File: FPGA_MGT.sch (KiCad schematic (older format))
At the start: 5 parts, among them U1 XC7K160T-FFG676

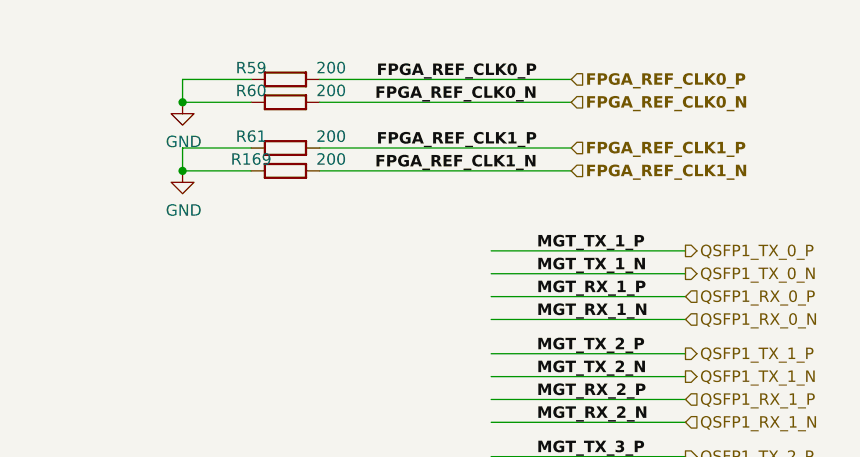
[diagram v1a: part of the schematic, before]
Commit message: REF CLK for MIG
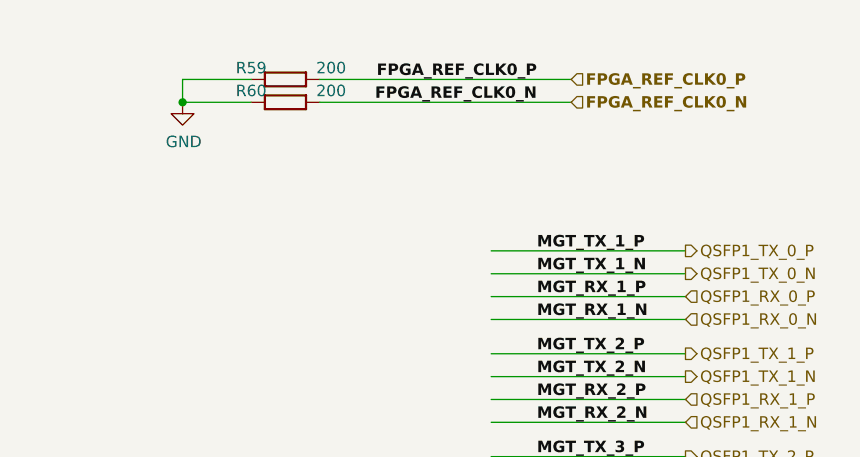
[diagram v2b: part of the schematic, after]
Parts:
- removed R169, R61: R0201_100R_1%_0.05W_200PPM, RESC0603X28N, symbol Resistors_SMD:R0201_100R_1%_0.05W_200PPM
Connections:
- net labels removed: FPGA_REF_CLK1_N, FPGA_REF_CLK1_P
- wire segments 148 -> 143
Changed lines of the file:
@@
 Comment4 ""
 $EndDescr
-Text HLabel 9700 1200 2    50   Input ~ 10
-FPGA_REF_CLK1_N
-Text HLabel 9700 1100 2    50   Input ~ 10
-FPGA_REF_CLK1_P
 Text HLabel 9700 900  2    50   Input ~ 10
 FPGA_REF_CLK0_N
@@
 Text Label 9550 900  2    50   ~ 10
 FPGA_REF_CLK0_N
-Text Label 9550 1100 2    50   ~ 10
-FPGA_REF_CLK1_P
-Text Label 9550 1200 2    50   ~ 10
-FPGA_REF_CLK1_N
 Wire Wire Line
 	8600 800  9700 800
@@
 	8600 900  9700 900
 Wire Wire Line
-	8600 1100 9700 1100
-Wire Wire Line
-	8600 1200 9700 1200
-Wire Wire Line
 	8000 800  8000 900
-Wire Wire Line
-	8000 1100 8000 1200
 $Comp
 L power:GND #PWR?
@@
 	1    0    0    -1
 $EndComp
-$Comp
-L power:GND #PWR?
-U 1 1 5FFB2211
-P 8000 1200
-AR Path="/5BD32060/5FFB2211" Ref="#PWR?"  Part="1"
-AR Path="/5BABAC65/5FFB2211" Ref="#PWR?"  Part="1"
-AR Path="/5CC24E97/5FFB2211" Ref="#PWR?"  Part="1"
-AR Path="/5CC393D3/5FFB2211" Ref="#PWR?"  Part="1"
-AR Path="/5CC6DBF7/5FFB2211" Ref="#PWR?"  Part="1"
-AR Path="/5CC8AFE1/5FFB2211" Ref="#PWR?"  Part="1"
-AR Path="/5C907554/5C417BCB/5FFB2211" Ref="#PWR?"  Part="1"
-AR Path="/5C907554/5DCA928C/5FFB2211" Ref="#PWR0494"  Part="1"
-F 0 "#PWR0494" H 8000 950 50  0001 C CNN
-F 1 "GND" H 8005 1027 50  0000 C CNN
-F 2 "" H 8000 1200 50  0001 C CNN
-F 3 "" H 8000 1200 50  0001 C CNN
-	1    8000 1200
-	1    0    0    -1
-$EndComp
 Wire Wire Line
 	8000 800  8300 800
@@
 	8000 900  8300 900
 Connection ~ 8000 900
-Wire Wire Line
-	8000 1100 8300 1100
-Wire Wire Line
-	8000 1200 8300 1200
-Connection ~ 8000 1200
 $Comp
 L Resistors_SMD:R0201_100R_1%_0.05W_200PPM R59
@@
 	1    0    0    -1
 $EndComp
-$Comp
-L Resistors_SMD:R0201_100R_1%_0.05W_200PPM R61
-U 1 1 5DCB78D4
-P 8300 1100
-F 0 "R61" H 8300 1150 50  0000 C CNN
-F 1 "R0201_100R_1%_0.05W_200PPM" H 8300 890 60  0001 L CNN
-F 2 "RESC0603X28N" H 8300 80  60  0001 L CNN
-F 3 "\\\\cern.ch\\dfs\\Applications\\Altium\\Datasheets\\R0201_VISHAY_CRCW e3.pdf" H 8300 710 60  0001 L CNN
-F 4 "200" H 8650 1150 50  0000 C CNN "~"
-F 5 "R0201_200R_1%_0.05W_200PPM" H 8300 620 60  0001 L CNN "Part Number"
-F 6 "Resistor - 1%" H 8300 530 60  0001 L CNN "Library Ref"
-F 7 "SchLib\\Resistors.SchLib" H 8300 440 60  0001 L CNN "Library Path"
-F 8 "=Value" H 8300 350 60  0001 L CNN "Comment"
-F 9 "Standard" H 8300 260 60  0001 L CNN "Component Kind"
-F 10 "Standard" H 8300 170 60  0001 L CNN "Component Type"
-F 11 "~~" H 8300 -10 60  0001 L CNN "PackageDescription"
-F 12 "2" H 8300 -100 60  0001 L CNN "Pin Count"
-F 13 "PcbLib\\Resistors SMD.PcbLib" H 8300 -190 60  0001 L CNN "Footprint Path"
-F 14 "RESC0603X28N" H 8300 -280 60  0001 L CNN "Footprint Ref"
-F 15 "100" H 8300 -370 60  0001 L CNN "Val"
-F 16 "Not Recommended" H 8300 -460 60  0001 L CNN "Status"
-F 17 "0.05W" H 8300 -550 60  0001 L CNN "Power"
-F 18 "±200ppm/°C" H 8300 -640 60  0001 L CNN "TC"
-F 19 "~~" H 8300 -730 60  0001 L CNN "Voltage"
-F 20 "±1%" H 8300 -820 60  0001 L CNN "Tolerance"
-F 21 "Thick Film Chip Resistor" H 8300 -910 60  0001 L CNN "Part Description"
-F 22 "GENERIC" H 8300 -1000 60  0001 L CNN "Manufacturer"
-F 23 "R0201_200R_1%_0.05W_200PPM" H 8300 -1090 60  0001 L CNN "Manufacturer Part Number"
-F 24 "0201" H 8300 -1180 60  0001 L CNN "Case"
-F 25 "No" H 8300 -1270 60  0001 L CNN "PressFit"
-F 26 "Yes" H 8300 -1360 60  0001 L CNN "Mounted"
-F 27 "~~" H 8300 -1450 60  0001 L CNN "Sense Comment"
-F 28 "No" H 8300 -1540 60  0001 L CNN "Sense"
-F 29 "~~" H 8300 -1630 60  0001 L CNN "Status Comment"
-F 30 "No" H 8300 -1720 60  0001 L CNN "Socket"
-F 31 "Yes" H 8300 -1810 60  0001 L CNN "SMD"
-F 32 "~~" H 8300 -1900 60  0001 L CNN "ComponentHeight"
-F 33 "VISHAY" H 8300 -1990 60  0001 L CNN "Manufacturer1 Example"
-F 34 "CRCW0201200RFNED" H 8300 -2080 60  0001 L CNN "Manufacturer1 Part Number"
-F 35 "0.27mm" H 8300 -2170 60  0001 L CNN "Manufacturer1 ComponentHeight"
-F 36 "\\\\cern.ch\\dfs\\Applications\\Altium\\Datasheets\\R0201_VISHAY_CRCW e3.pdf" H 8300 -2260 60  0001 L CNN "HelpURL"
-F 37 "CERN DEM JLC" H 8300 -2350 60  0001 L CNN "Author"
-F 38 "11/13/14 00:00:00" H 8300 -2440 60  0001 L CNN "CreateDate"
-F 39 "11/13/14 00:00:00" H 8300 -2530 60  0001 L CNN "LatestRevisionDate"
-F 40 "Resistors SMD" H 8300 -2620 60  0001 L CNN "Library Name"
-F 41 "This work is licensed under the Creative Commons CC-BY-SA 4.0 License. To the extent that circuit schematics that use Licensed Material can be considered to be ‘Adapted Material’, then the copyright holder waives article 3.b of the license with respect to these schematics." H 8300 -2710 60  0001 L CNN "License"
-	1    8300 1100
-	1    0    0    -1
-$EndComp
-$Comp
-L Resistors_SMD:R0201_100R_1%_0.05W_200PPM R169
-U 1 1 5DCC9ABA
-P 8300 1200
-F 0 "R169" H 8300 1250 50  0000 C CNN
-F 1 "R0201_100R_1%_0.05W_200PPM" H 8300 990 60  0001 L CNN
-F 2 "RESC0603X28N" H 8300 180 60  0001 L CNN
-F 3 "\\\\cern.ch\\dfs\\Applications\\Altium\\Datasheets\\R0201_VISHAY_CRCW e3.pdf" H 8300 810 60  0001 L CNN
-F 4 "200" H 8650 1250 50  0000 C CNN "~"
-F 5 "R0201_200R_1%_0.05W_200PPM" H 8300 720 60  0001 L CNN "Part Number"
-F 6 "Resistor - 1%" H 8300 630 60  0001 L CNN "Library Ref"
-F 7 "SchLib\\Resistors.SchLib" H 8300 540 60  0001 L CNN "Library Path"
-F 8 "=Value" H 8300 450 60  0001 L CNN "Comment"
-F 9 "Standard" H 8300 360 60  0001 L CNN "Component Kind"
-F 10 "Standard" H 8300 270 60  0001 L CNN "Component Type"
-F 11 "~~" H 8300 90  60  0001 L CNN "PackageDescription"
-F 12 "2" H 8300 0   60  0001 L CNN "Pin Count"
-F 13 "PcbLib\\Resistors SMD.PcbLib" H 8300 -90 60  0001 L CNN "Footprint Path"
-F 14 "RESC0603X28N" H 8300 -180 60  0001 L CNN "Footprint Ref"
-F 15 "100" H 8300 -270 60  0001 L CNN "Val"
-F 16 "Not Recommended" H 8300 -360 60  0001 L CNN "Status"
-F 17 "0.05W" H 8300 -450 60  0001 L CNN "Power"
-F 18 "±200ppm/°C" H 8300 -540 60  0001 L CNN "TC"
-F 19 "~~" H 8300 -630 60  0001 L CNN "Voltage"
-F 20 "±1%" H 8300 -720 60  0001 L CNN "Tolerance"
-F 21 "Thick Film Chip Resistor" H 8300 -810 60  0001 L CNN "Part Description"
-F 22 "GENERIC" H 8300 -900 60  0001 L CNN "Manufacturer"
-F 23 "R0201_200R_1%_0.05W_200PPM" H 8300 -990 60  0001 L CNN "Manufacturer Part Number"
-F 24 "0201" H 8300 -1080 60  0001 L CNN "Case"
-F 25 "No" H 8300 -1170 60  0001 L CNN "PressFit"
-F 26 "Yes" H 8300 -1260 60  0001 L CNN "Mounted"
-F 27 "~~" H 8300 -1350 60  0001 L CNN "Sense Comment"
-F 28 "No" H 8300 -1440 60  0001 L CNN "Sense"
-F 29 "~~" H 8300 -1530 60  0001 L CNN "Status Comment"
-F 30 "No" H 8300 -1620 60  0001 L CNN "Socket"
-F 31 "Yes" H 8300 -1710 60  0001 L CNN "SMD"
-F 32 "~~" H 8300 -1800 60  0001 L CNN "ComponentHeight"
-F 33 "VISHAY" H 8300 -1890 60  0001 L CNN "Manufacturer1 Example"
-F 34 "CRCW0201200RFNED" H 8300 -1980 60  0001 L CNN "Manufacturer1 Part Number"
-F 35 "0.27mm" H 8300 -2070 60  0001 L CNN "Manufacturer1 ComponentHeight"
-F 36 "\\\\cern.ch\\dfs\\Applications\\Altium\\Datasheets\\R0201_VISHAY_CRCW e3.pdf" H 8300 -2160 60  0001 L CNN "HelpURL"
-F 37 "CERN DEM JLC" H 8300 -2250 60  0001 L CNN "Author"
-F 38 "11/13/14 00:00:00" H 8300 -2340 60  0001 L CNN "CreateDate"
-F 39 "11/13/14 00:00:00" H 8300 -2430 60  0001 L CNN "LatestRevisionDate"
-F 40 "Resistors SMD" H 8300 -2520 60  0001 L CNN "Library Name"
-F 41 "This work is licensed under the Creative Commons CC-BY-SA 4.0 License. To the extent that circuit schematics that use Licensed Material can be considered to be ‘Adapted Material’, then the copyright holder waives article 3.b of the license with respect to these schematics." H 8300 -2610 60  0001 L CNN "License"
-	1    8300 1200
-	1    0    0    -1
-$EndComp
